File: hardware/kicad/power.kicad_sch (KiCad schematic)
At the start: 19 parts, among them Q2 PMV32UP, Q7 DMG1012UW, U10 RT9080-33GJ5, U12 RT9193, U3 TPS22917DBVR, U8 XC6215B332MR-G

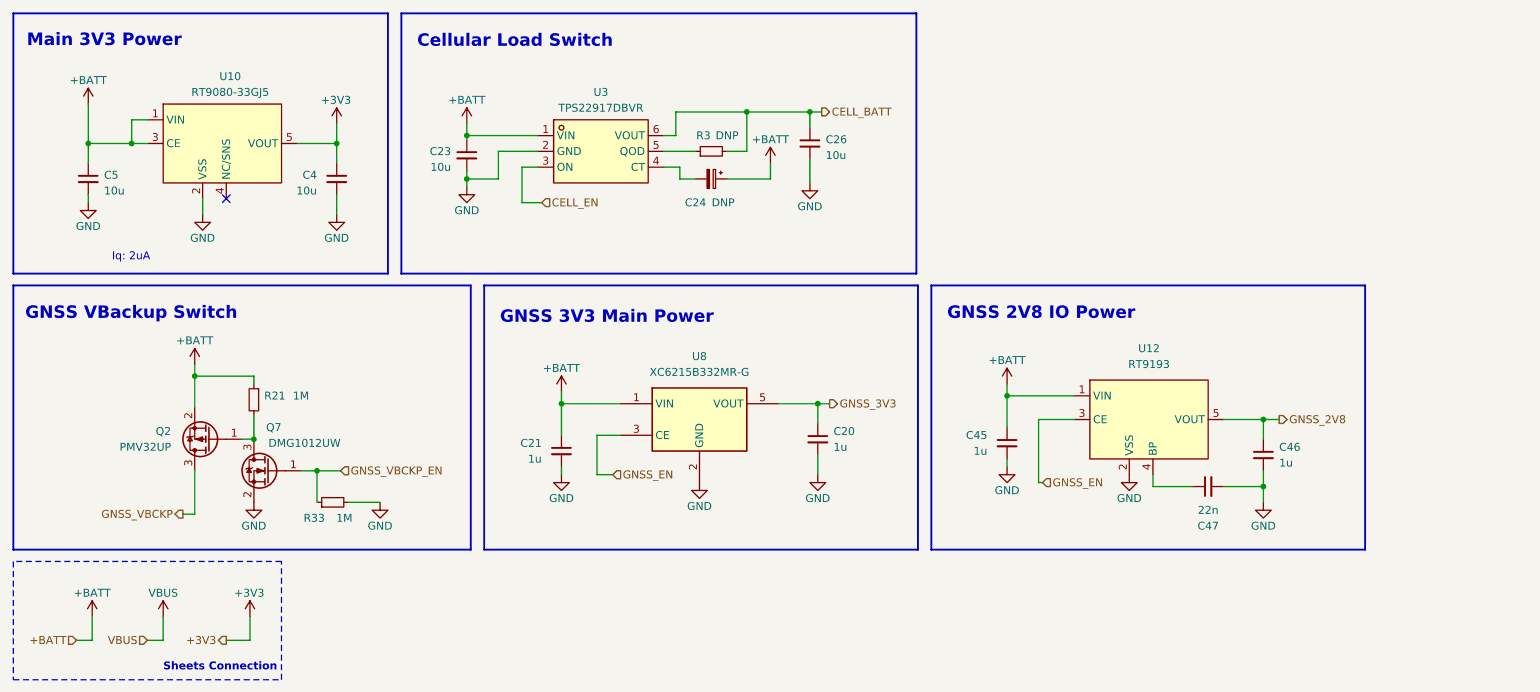
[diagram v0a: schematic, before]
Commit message: Added Ignion Antenna
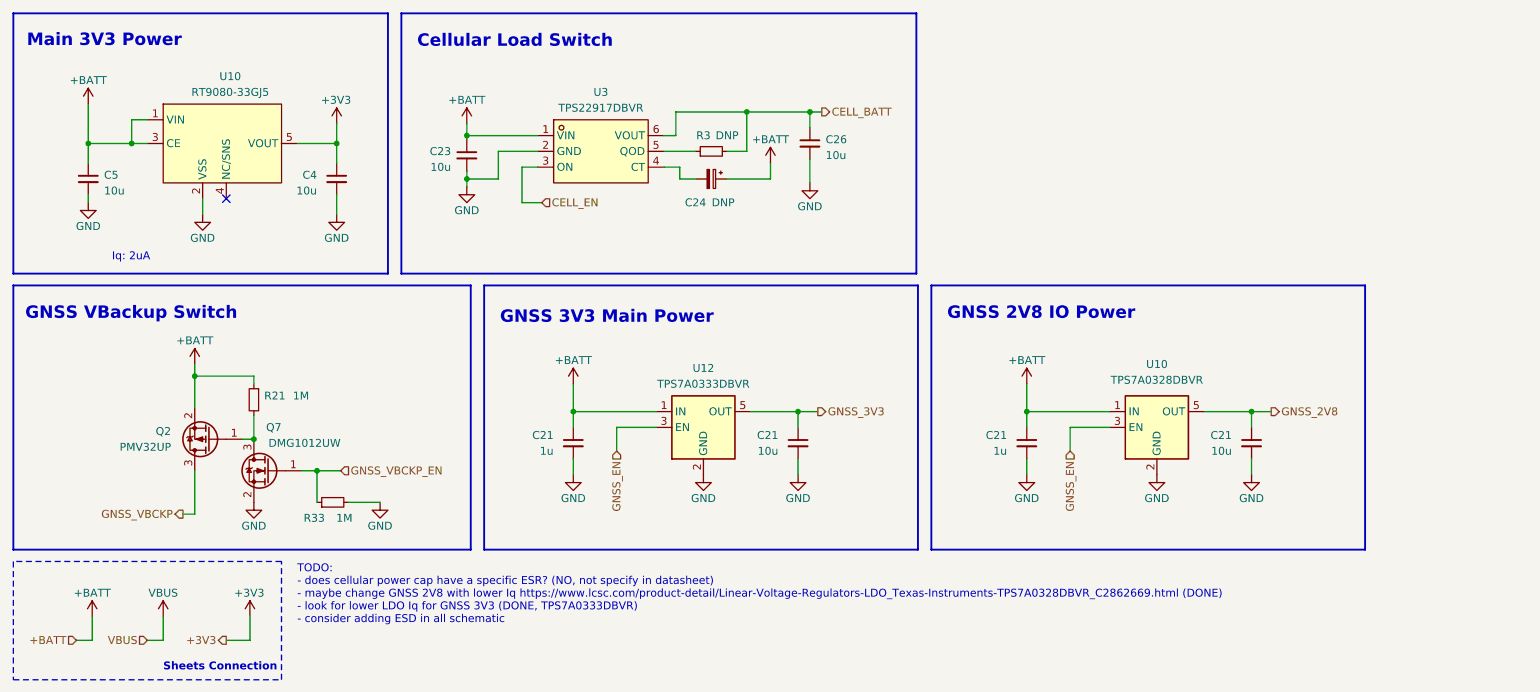
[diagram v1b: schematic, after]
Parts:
- removed C20, C21, C45, C46: 1u, Capacitor_SMD:C_0603_1608Metric, symbol Device:C_Small
- removed C47: 22n, Capacitor_SMD:C_0603_1608Metric, symbol Device:C_Small
- removed U12: RT9193, Package_TO_SOT_SMD:SOT-23-5_HandSoldering, symbol bwlc1a:RT9193
- removed U8: XC6215B332MR-G, Package_TO_SOT_SMD:SOT-23-5, symbol Regulator_Linear:XC6210B332MR
- added C21 (x2): 10u, Capacitor_SMD:C_0603_1608Metric, symbol Device:C_Small
- added C21 (x2): 1u, Capacitor_SMD:C_0603_1608Metric, symbol Device:C_Small
- added U10: TPS7A0328DBVR, Package_TO_SOT_SMD:SOT-23-5, symbol Regulator_Linear:TPS7A0508PDBV
- added U12: TPS7A0333DBVR, Package_TO_SOT_SMD:SOT-23-5, symbol Regulator_Linear:TPS7A0508PDBV
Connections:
- net +BATT: now also C21.1, C21.1, U10.1 (IN), U12.1 (IN)
- net GND: now also C21.2, C21.2, C21.2, C21.2, U10.2 (GND), U12.2 (GND)
- net GNSS_2V8: now also C21.1, U10.5 (OUT)
- net GNSS_3V3: now also C21.1, U12.5 (OUT)
- net GNSS_EN: now also U10.3 (EN), U12.3 (EN)
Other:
- note added: "TODO: - does cellular power cap have a specific ESR? (NO, not specify in datasheet) - maybe change GNSS 2V8 with lower Iq https://www.lcsc.com/product-detail/Linear-Voltage-Regulators-LDO_Texas-Instruments-TPS7A0328DBVR_C2862669.html (DONE) - look for lower LDO Iq for GNSS 3V3 (DONE, TPS7A0333DBVR) - consider adding ESD in all schematic"
